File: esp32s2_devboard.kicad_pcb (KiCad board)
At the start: 2 copper layers, 22.5 x 49.3 mm, 31 parts, among them J1 USB_C_Receptacle_USB2.0, J2 USB_C_Receptacle_USB2.0, J3 Conn_01x15, J4 Conn_01x15, Q1 BC817, Q2 BC817, SW1 SW_DPST, SW2 SW_DPST, U1 ESP32-S2-MINI-2, U2 AP2112K-3.3, U3 CH340C

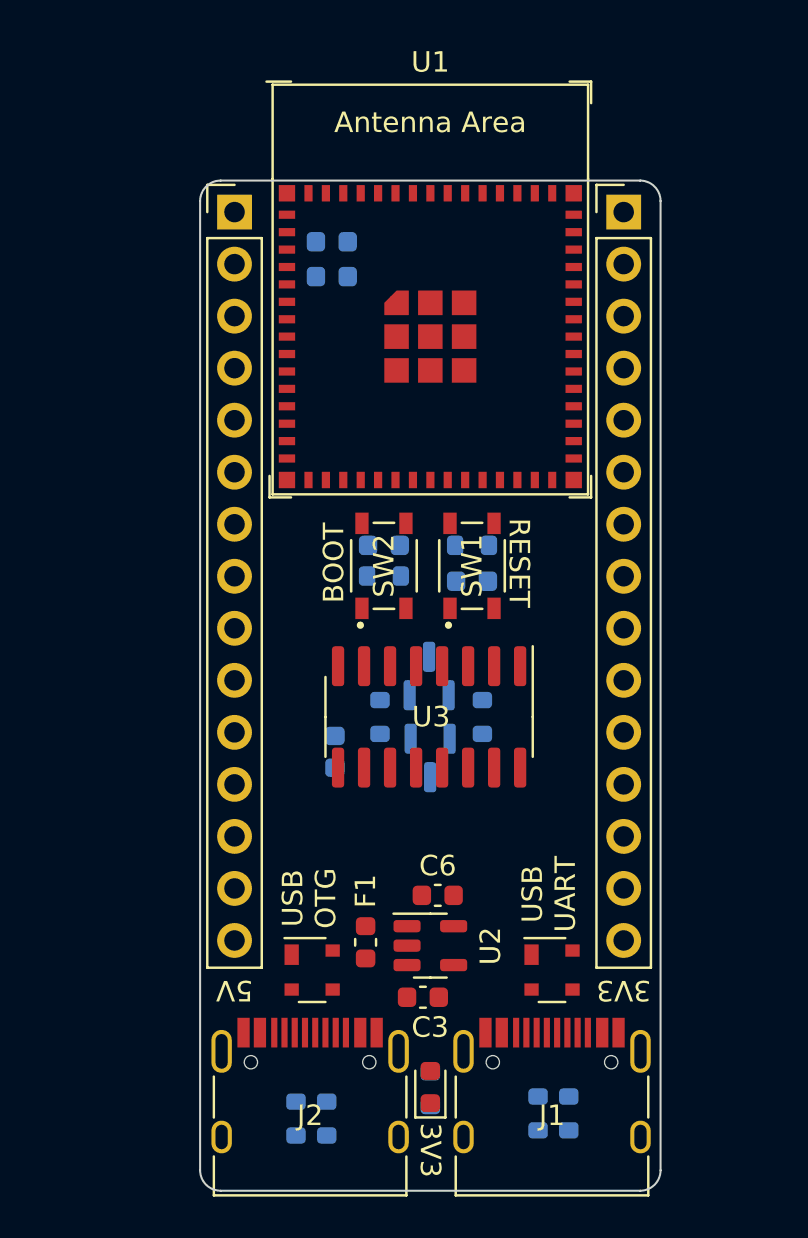
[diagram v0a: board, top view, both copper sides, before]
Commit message: Added sch scheets, project on hold
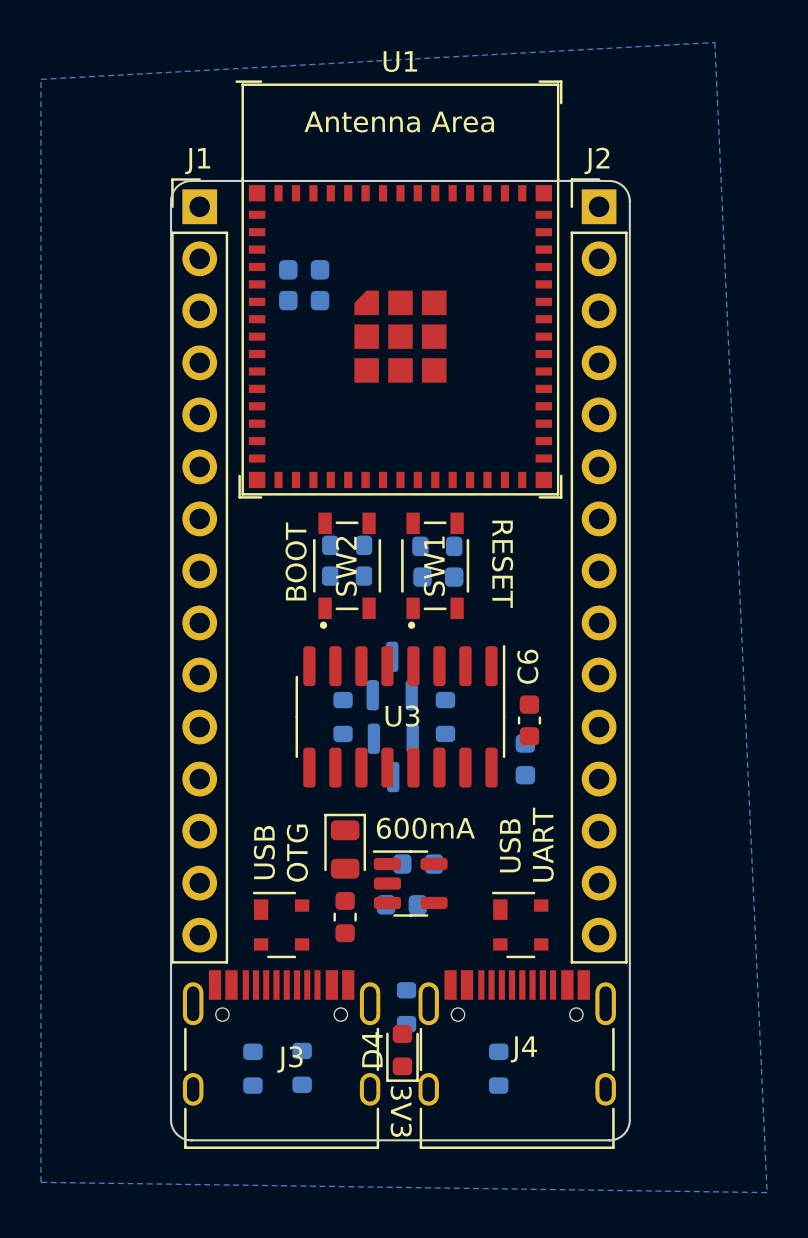
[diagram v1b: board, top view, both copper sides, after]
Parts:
- added D4: GREEN, LED_SMD:LED_0603_1608Metric, F.Cu at (161.2, 90.7)
- C1: value 22uF -> 1u
- C2, C5: value 100n -> 1u
- C3: value 1u -> 22uF; moved to B.Cu
- C4, C7: value 1u -> 100n
- D1: value PRTR5V0U2X -> D_Schottky; footprint Package_TO_SOT_SMD:SOT-143 -> Diode_SMD:D_0805_2012Metric
- D3: value GREEN -> PRTR5V0U2X; footprint LED_SMD:LED_0603_1608Metric -> Package_TO_SOT_SMD:SOT-143
- J1, J2: value USB_C_Receptacle_USB2.0 -> Conn_01x15; footprint Connector_USB:USB_C_Receptacle_HRO_TYPE-C-31-M-12 -> Connector_PinHeader_2.54mm:PinHeader_1x15_P2.54mm_Vertical
- J3, J4: value Conn_01x15 -> USB_C_Receptacle_USB2.0; footprint Connector_PinHeader_2.54mm:PinHeader_1x15_P2.54mm_Vertical -> Connector_USB:USB_C_Receptacle_HRO_TYPE-C-31-M-12
- R1: value 5k1 -> 3k3
- R2, R3: value 5k1 -> 22k
- R5, R7: value 22k -> 5k1
- R6: value 3k3 -> 5k1
- moved J1 47.6 mm to (151.3, 49.5)
- moved J2 46.6 mm to (170.8, 49.5)
- moved J4 42.1 mm to (166.8, 91.6)
- moved J3 41.8 mm to (155.3, 91.6)
- moved C3 34.5 mm to (156.4, 54.1), turned to 180 degrees
- moved C1 32.6 mm to (161.2, 83.6), turned to 0 degrees
- moved C2 29.0 mm to (162.0, 81.6), turned to 180 degrees
- moved R2 28.4 mm to (162.9, 66.1), turned to 0 degrees
- moved R3 28.1 mm to (158.5, 66.1), turned to 0 degrees
- moved R5 27.7 mm to (153.9, 91.6), turned to -90 degrees
- moved C4 17.3 mm to (156.4, 52.6)
- moved C7 12.5 mm to (167.2, 76.5), turned to 90 degrees
- moved D1 11.7 mm to (158.4, 80.9), turned to -90 degrees
- moved C5 9.91 mm to (162.9, 67.6), turned to 180 degrees
- moved C6 9.64 mm to (167.4, 74.6), turned to -90 degrees
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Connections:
- net /DTR renamed /Pheripherals/DTR
- net /IO15 renamed /MCU/IO15
- net /IO16 renamed /MCU/IO16
- net /IO39 renamed /MCU/IO39
- net /IO40 renamed /MCU/IO40
- net /IO41 renamed /MCU/IO41
- net /IO42 renamed /MCU/IO42
- net /RTS renamed /Pheripherals/RTS
- C1 pad 1: GND -> +5V
- C1 pad 2: +3V3 -> GND
- C3 pad 1: +5V -> GND
- C3 pad 2: GND -> +3V3
- C4 pad 1: RESET -> +3V3
- C5 pad 1: +3V3 -> RESET
- C6 pad 1: +3V3 -> GPIO0
- C7 pad 1: GPIO0 -> +3V3
- D1 pad 1: GND -> +5V
- D1 pad 2: unconnected-(D1-Pad2) -> Net-(D1-Pad2)
- D2 pad 2: /UART_USB_D- -> /Pheripherals/UART_USB_D-
- D2 pad 3: /UART_USB_D+ -> /Pheripherals/UART_USB_D+
- D3 pad 2: Net-(D3-Pad2) -> /Pheripherals/OTG_USB_D-
- F1 pad 1: /VBUS -> /Power/VBUS
- F1 pad 2: +5V -> Net-(D1-Pad2)
- R1 pad 1: Net-(J1-PadA5) -> +3V3
- R1 pad 2: GND -> Net-(D4-Pad2)
- R2 pad 1: Net-(J1-PadB5) -> +3V3
- R2 pad 2: GND -> RESET
- R3 pad 1: Net-(J2-PadA5) -> +3V3
- R3 pad 2: GND -> GPIO0
- R4 pad 1: Net-(J2-PadB5) -> Net-(J3-PadA5)
- R5 pad 1: +3V3 -> Net-(J3-PadB5)
- R5 pad 2: RESET -> GND
- R6 pad 1: +3V3 -> Net-(J4-PadA5)
- R6 pad 2: Net-(D3-Pad2) -> GND
- R7 pad 1: +3V3 -> Net-(J4-PadB5)
- R7 pad 2: GPIO0 -> GND
- U1 pad 10: /IO6 -> /MCU/IO6
- U1 pad 11: /IO7 -> /MCU/IO7
- U1 pad 12: /IO8 -> /MCU/IO8
- U1 pad 13: /IO9 -> /MCU/IO9
- U1 pad 14: /IO10 -> /MCU/IO10
- U1 pad 15: /IO11 -> /MCU/IO11
- U1 pad 16: /IO12 -> /MCU/IO12
- U1 pad 17: /IO13 -> /MCU/IO13
- U1 pad 18: /IO14 -> /MCU/IO14
- U1 pad 21: /IO17 -> /MCU/IO17
- U1 pad 22: /IO18 -> /MCU/IO18
- U1 pad 25: unconnected-(U1-Pad25) -> /MCU/IO21
- U1 pad 26: unconnected-(U1-Pad26) -> /MCU/IO26
- U1 pad 28: unconnected-(U1-Pad28) -> /MCU/IO33
- U1 pad 29: unconnected-(U1-Pad29) -> /MCU/IO34
- U1 pad 31: unconnected-(U1-Pad31) -> /MCU/IO35
- U1 pad 32: unconnected-(U1-Pad32) -> /MCU/IO36
- U1 pad 33: unconnected-(U1-Pad33) -> /MCU/IO37
- U1 pad 34: unconnected-(U1-Pad34) -> /MCU/IO38
- U1 pad 5: /IO1 -> /MCU/IO1
- U1 pad 6: /IO2 -> /MCU/IO2
- U1 pad 7: /IO3 -> /MCU/IO3
- U1 pad 8: /IO4 -> /MCU/IO4
- U1 pad 9: /IO5 -> /MCU/IO5
- U3 pad 5: /UART_USB_D+ -> /Pheripherals/UART_USB_D+
- U3 pad 6: /UART_USB_D- -> /Pheripherals/UART_USB_D-
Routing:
- added copper zone on B.Cu, net GND
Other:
- board size 22.5 x 49.3 mm -> 22.4 x 46.8 mm
- board text added: "600mA"
- board text removed: "5V"
